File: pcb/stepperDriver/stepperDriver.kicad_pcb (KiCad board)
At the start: 2 copper layers, 18 parts, among them IC1 ATTINY84-P, P1 CONN_6, P2 CONN_7, U1 L298D

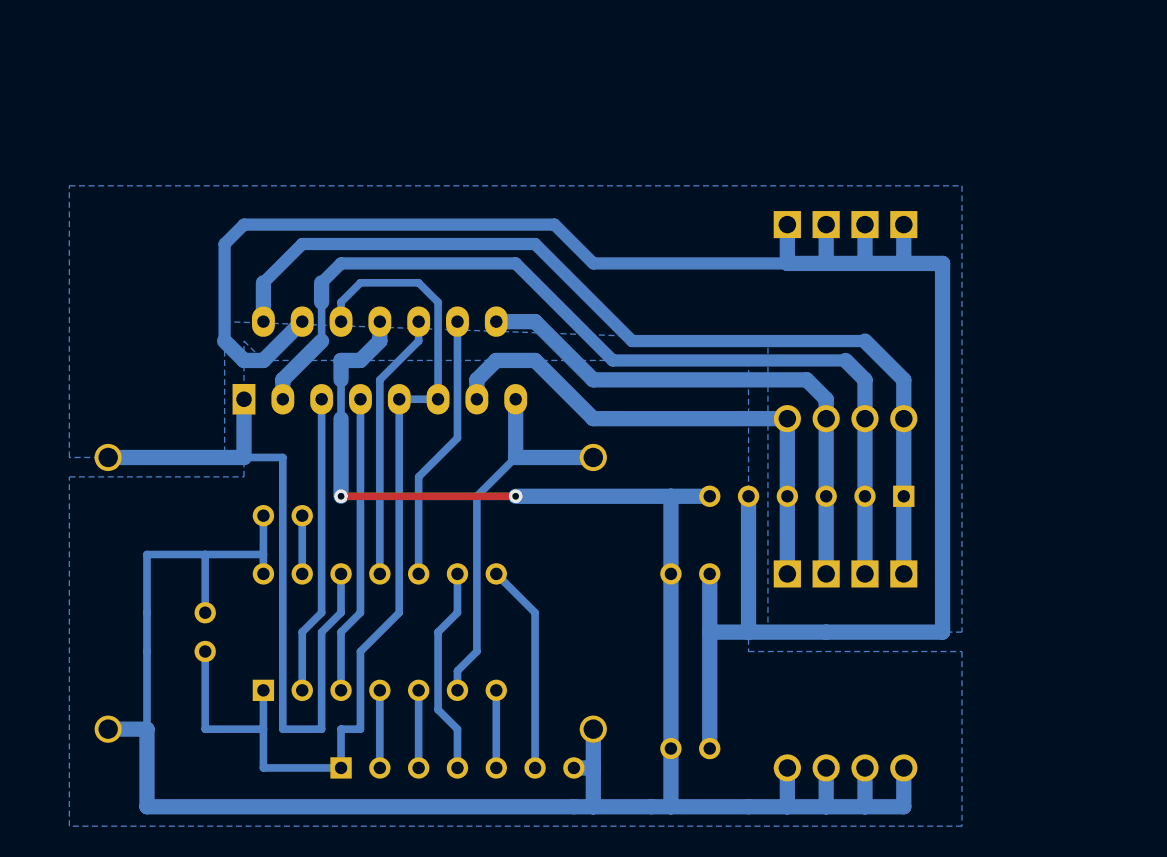
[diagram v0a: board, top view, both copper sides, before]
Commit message: group of pcb
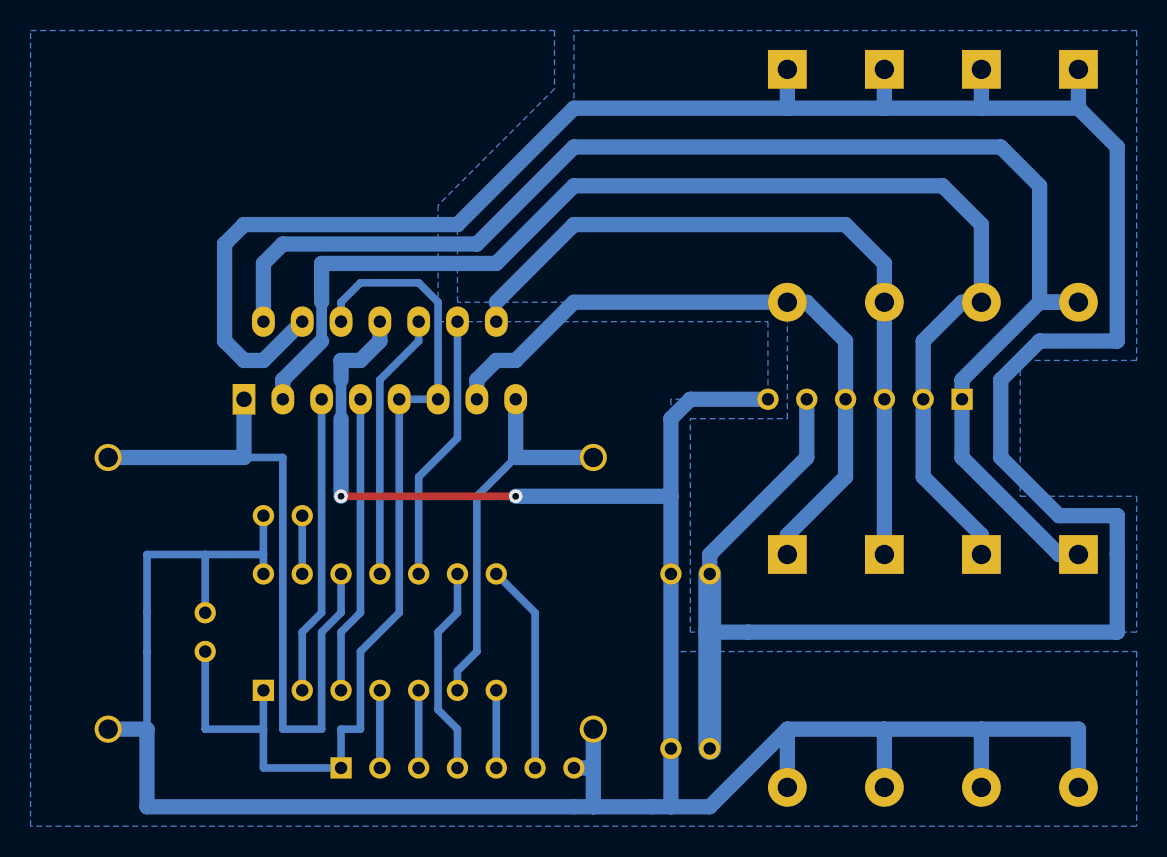
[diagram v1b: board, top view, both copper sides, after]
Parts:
- D1, D2, D3, D4, D5, D6, D7, D8: footprint D5 -> D6
- moved D1 14.5 mm to (116.8, 44.5)
- moved D2 11.7 mm to (110.5, 44.5)
- moved D5 11.4 mm to (116.8, 76.2)
- moved D4 9.67 mm to (104.1, 44.5)
- moved D3 8.89 mm to (97.8, 44.5)
- moved D6 7.62 mm to (110.5, 76.2)
- moved P1 7.41 mm to (102.9, 58.4)
- moved D8 3.81 mm to (104.1, 76.2)
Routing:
- net N-0000019: track 134.0 -> 181.8 mm
- net N-000003: track 61.9 -> 94.0 mm
- net GND: track 158.0 -> 186.0 mm
- net N-000004: track 60.6 -> 81.8 mm
- net N-000006: track 35.1 -> 48.9 mm
- net N-000005: track 33.9 -> 44.1 mm
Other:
- net class Default: clearance 0.254 -> 0.16
- rule trace_clearance: 0.254 -> 0.16
